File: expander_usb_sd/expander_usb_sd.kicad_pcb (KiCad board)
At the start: 2 copper layers, 59.7 x 128.5 mm, 10 parts, among them J1 Micro_SD_Card_Det1, J2 Internal_USB_Host_Teensy, J2-USBHostPower1 USB power - host

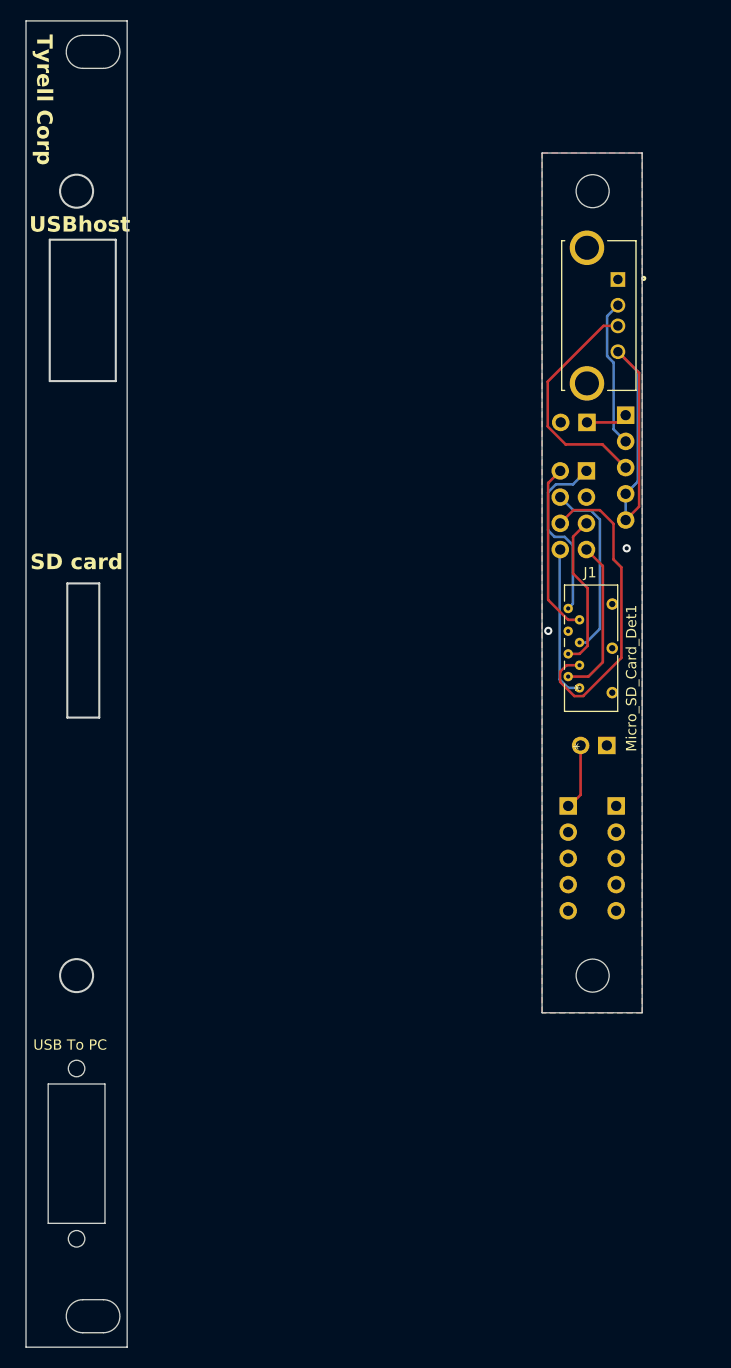
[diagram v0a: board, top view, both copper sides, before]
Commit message: fucking connect the USB Host pins that were completely unconnected previously... facepalm!
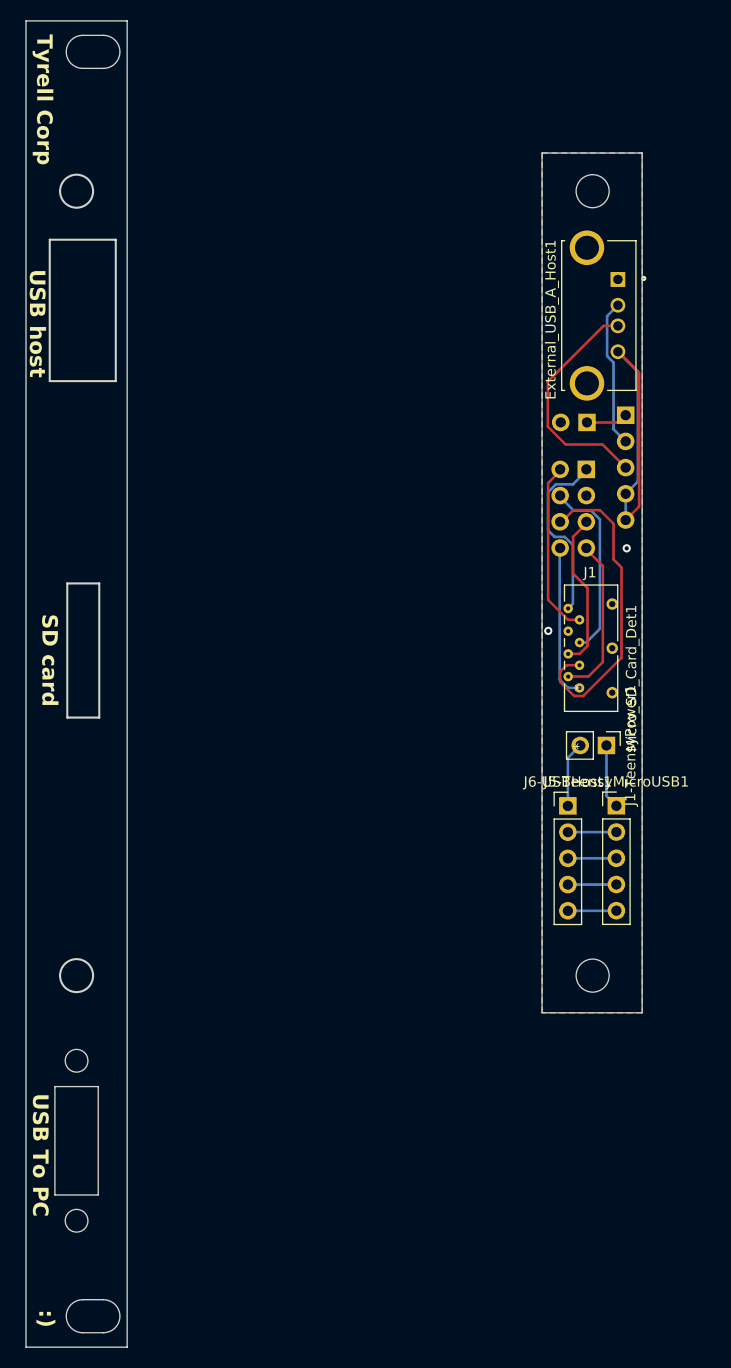
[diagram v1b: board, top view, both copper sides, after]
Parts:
- removed SD: Conn_02x04_Odd_Even, Connector_PinHeader_2.54mm:PinHeader_2x04_P2.54mm_Vertical
- removed TeensyMicroUSB-C: USB 5 pin to Teensy/MicroUSB, Connector_PinHeader_2.54mm:PinHeader_1x05_P2.54mm_Vertical
- removed TeensyPower: USB power - Teensy device, Connector_PinHeader_2.54mm:PinHeader_1x02_P2.54mm_Vertical
- removed USBHost-A: USB 5 pin to frontpanel/Type C, Connector_PinHeader_2.54mm:PinHeader_1x05_P2.54mm_Vertical
- added J1-TeensyPower1: USB power - Teensy device, Connector_PinHeader_2.54mm:PinHeader_1x02_P2.54mm_Vertical, F.Cu at (130.5, 108.3)
- added J5-TeensyMicroUSB1: USB 5 pin to Teensy/MicroUSB, Connector_PinHeader_2.54mm:PinHeader_1x05_P2.54mm_Vertical, F.Cu at (131.5, 114.2)
- added J6-USBHost1: USB 5 pin to frontpanel/Type C, Connector_PinHeader_2.54mm:PinHeader_1x05_P2.54mm_Vertical, F.Cu at (126.8, 114.2)
- added SD_connector1: Conn_02x04_Odd_Even, Connector_PinHeader_2.54mm:PinHeader_2x04_P2.54mm_Vertical, B.Cu at (128.6, 81.5)
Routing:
- net Net-(J1-TeensyPower1-Pin_1): track 0.00 -> 6.25 mm
- net Net-(J5-TeensyMicroUSB1-Pin_4): track 0.00 -> 4.70 mm
- net Net-(J5-TeensyMicroUSB1-Pin_2): track 0.00 -> 4.70 mm
- net Net-(J5-TeensyMicroUSB1-Pin_5): track 0.00 -> 4.70 mm
- net Net-(J5-TeensyMicroUSB1-Pin_3): track 0.00 -> 4.70 mm
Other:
- outline, holes or cut-outs redrawn
- board text added: ":)"
- board text added: "USB host"
- board text removed: "USBhost"

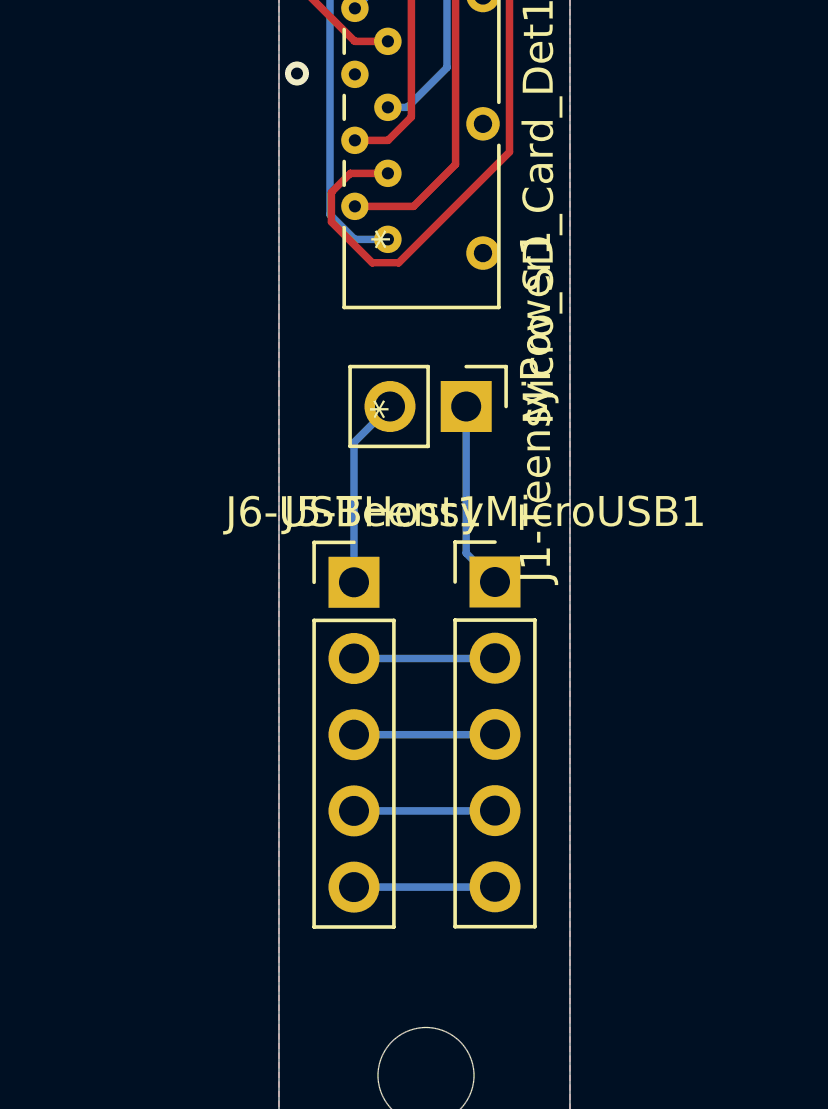
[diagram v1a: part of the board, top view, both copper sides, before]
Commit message: flip headers back to correct side of board
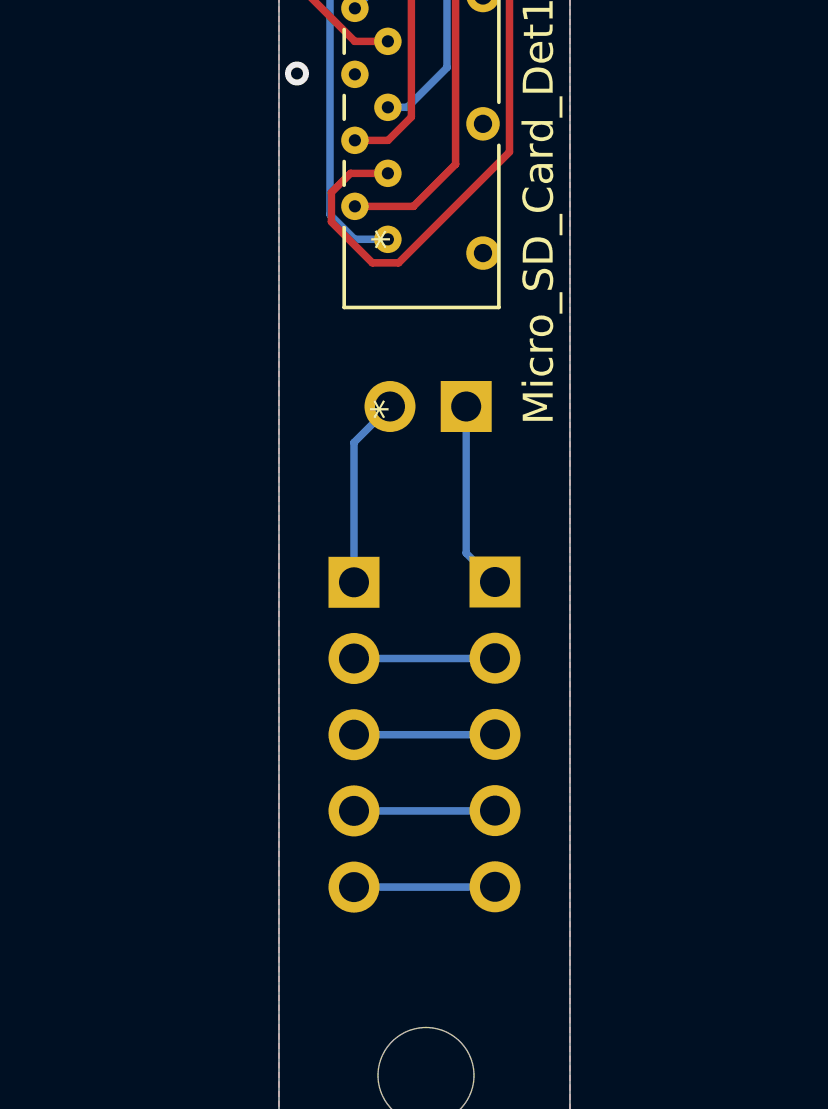
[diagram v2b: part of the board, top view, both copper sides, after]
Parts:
- J1-TeensyPower1, J5-TeensyMicroUSB1, J6-USBHost1: moved to B.Cu
- turned J1-TeensyPower1 to 90 degrees
- turned J5-TeensyMicroUSB1 to 180 degrees
- turned J6-USBHost1 to 180 degrees

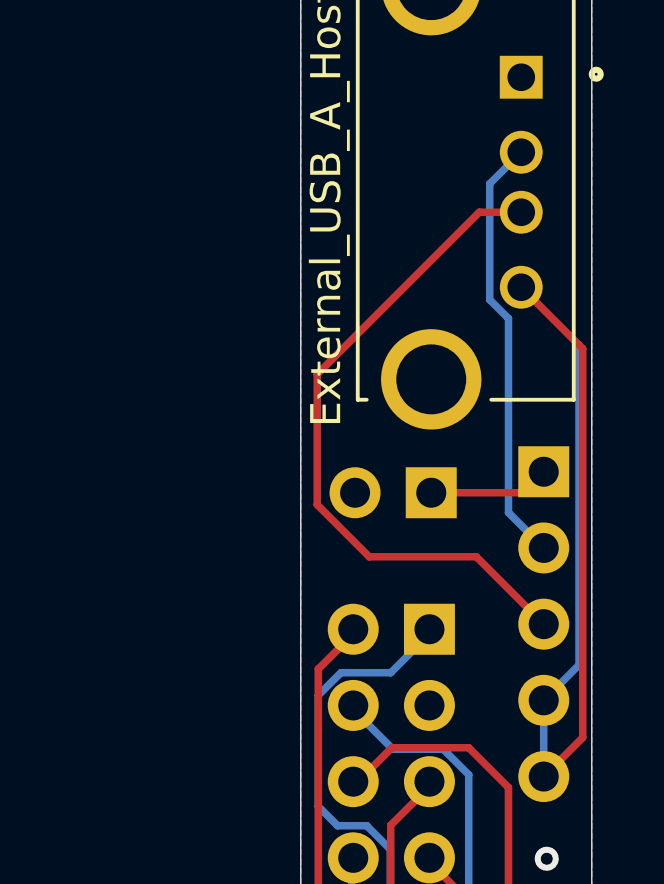
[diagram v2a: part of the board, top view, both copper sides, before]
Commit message: some improved routing
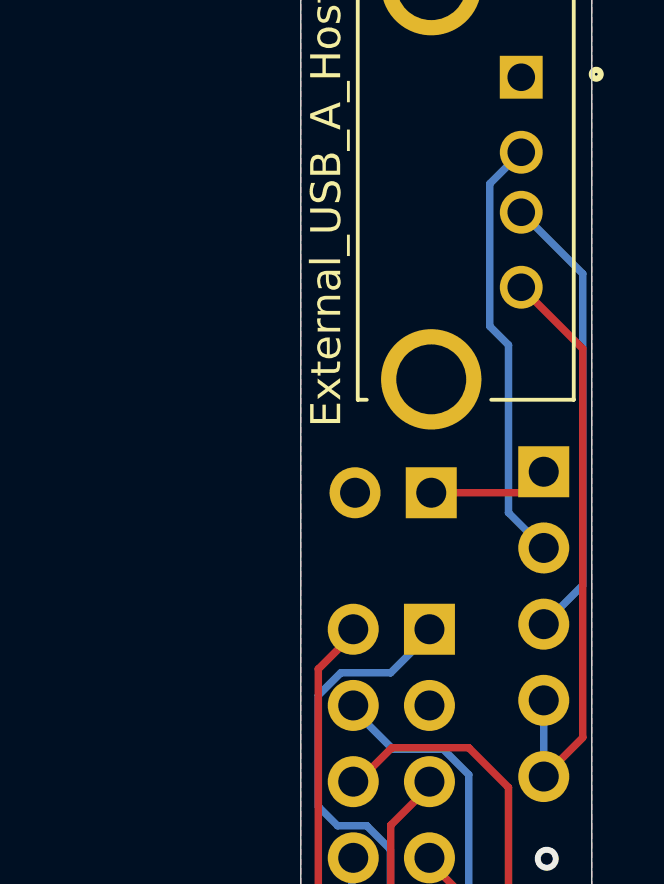
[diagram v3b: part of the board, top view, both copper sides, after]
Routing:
- net Net-(External_USB_A_Host1-GND): track 35.3 -> 20.2 mm
- net Net-(External_USB_A_Host1-D+): track 22.6 -> 15.1 mm
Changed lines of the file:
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@@
     )
   )
-  (segment (start 131.225 71.194368) (end 130.6 70.569368) (width 0.25) (layer "B.Cu") (net 2))
-  (segment (start 130.6 70.569368) (end 130.6 66.7) (width 0.25) (layer "B.Cu") (net 2))
-  (segment (start 131.225 77.665) (end 131.225 71.194368) (width 0.25) (layer "B.Cu") (net 2))
+  (segment (start 131.225 72.075) (end 130.6 71.45) (width 0.25) (layer "B.Cu") (net 2))
+  (segment (start 131.225 77.665) (end 131.225 72.075) (width 0.25) (layer "B.Cu") (net 2))
+  (segment (start 132.4 78.84) (end 131.225 77.665) (width 0.25) (layer "B.Cu") (net 2))
   (segment (start 130.6 66.7) (end 131.65 65.65) (width 0.25) (layer "B.Cu") (net 2))
-  (segment (start 132.4 78.84) (end 131.225 77.665) (width 0.25) (layer "B.Cu") (net 2))
-  (segment (start 126.583299 79.135) (end 124.85 77.401701) (width 0.25) (layer "F.Cu") (net 3))
-  (segment (start 124.85 77.401701) (end 124.85 73.05) (width 0.25) (layer "F.Cu") (net 3))
-  (segment (start 130.155 79.135) (end 126.583299 79.135) (width 0.25) (layer "F.Cu") (net 3))
-  (segment (start 130.25 67.65) (end 131.65 67.65) (width 0.25) (layer "F.Cu") (net 3))
-  (segment (start 132.4 81.38) (end 130.155 79.135) (width 0.25) (layer "F.Cu") (net 3))
-  (segment (start 124.85 73.05) (end 130.25 67.65) (width 0.25) (layer "F.Cu") (net 3))
+  (segment (start 130.6 71.45) (end 130.6 66.7) (width 0.25) (layer "B.Cu") (net 2))
+  (segment (start 133.7 80.08) (end 133.7 69.7) (width 0.25) (layer "B.Cu") (net 3))
+  (segment (start 133.7 69.7) (end 131.65 67.65) (width 0.25) (layer "B.Cu") (net 3))
+  (segment (start 132.4 81.38) (end 133.7 80.08) (width 0.25) (layer "B.Cu") (net 3))
   (segment (start 133.7 85.16) (end 133.7 72.2) (width 0.25) (layer "F.Cu") (net 4))
   (segment (start 133.7 72.2) (end 131.65 70.15) (width 0.25) (layer "F.Cu") (net 4))
   (segment (start 132.4 86.46) (end 133.7 85.16) (width 0.25) (layer "F.Cu") (net 4))
   (segment (start 132.4 83.92) (end 132.4 86.46) (width 0.25) (layer "B.Cu") (net 4))
-  (segment (start 133.575 72.075) (end 131.65 70.15) (width 0.25) (layer "B.Cu") (net 4))
-  (segment (start 133.575 82.745) (end 133.575 72.075) (width 0.25) (layer "B.Cu") (net 4))
-  (segment (start 132.4 83.92) (end 133.575 82.745) (width 0.25) (layer "B.Cu") (net 4))
   (segment (start 127.929999 102.728) (end 126.823801 102.728) (width 0.25) (layer "B.Cu") (net 5))
   (segment (start 126 101.904199) (end 126 89.38) (width 0.25) (layer "B.Cu") (net 5))
